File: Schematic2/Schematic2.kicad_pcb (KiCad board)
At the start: 2 copper layers, 100 x 119 mm, 52 parts, among them SW1 Rotary_Encoder_Switch, U1 Kailhlowprofile, U10 Kailhlowprofile, U11 Kailhlowprofile, U12 Kailhlowprofile, U13 Kailhlowprofile, U14 Kailhlowprofile, U15 Kailhlowprofile, U16 Kailhlowprofile, U17 Kailhlowprofile, U18 Kailhlowprofile, U19 Kailhlowprofile, U2 Kailhlowprofile, U20 Kailhlowprofile, U3 Kailhlowprofile, U4 Kailhlowprofile, U5 Kailhlowprofile, U6 Kailhlowprofile, U7 Kailhlowprofile, U8 Kailhlowprofile, U9 Kailhlowprofile

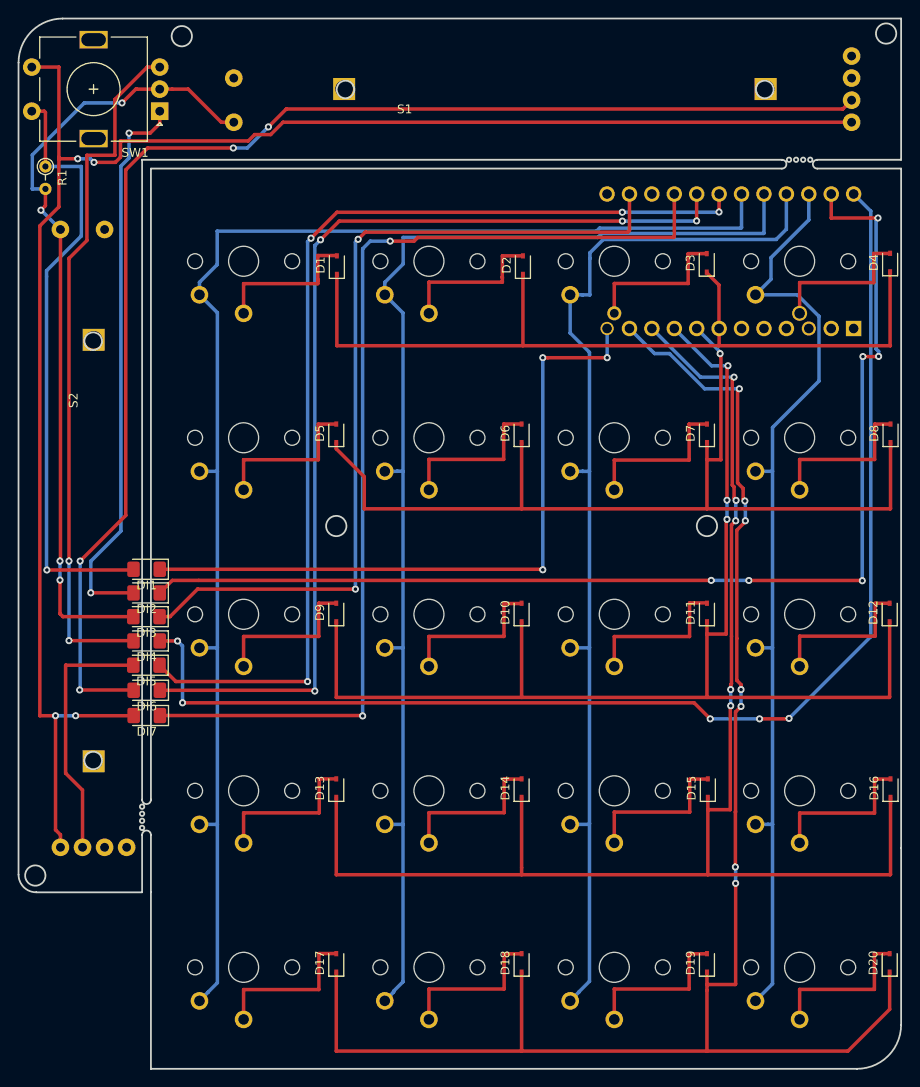
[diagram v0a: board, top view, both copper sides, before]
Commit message: Print time - final and absolutely done edition
This edition is completely done, for realz, and has all the files you need to print a macro keyboard with Kailh switches.
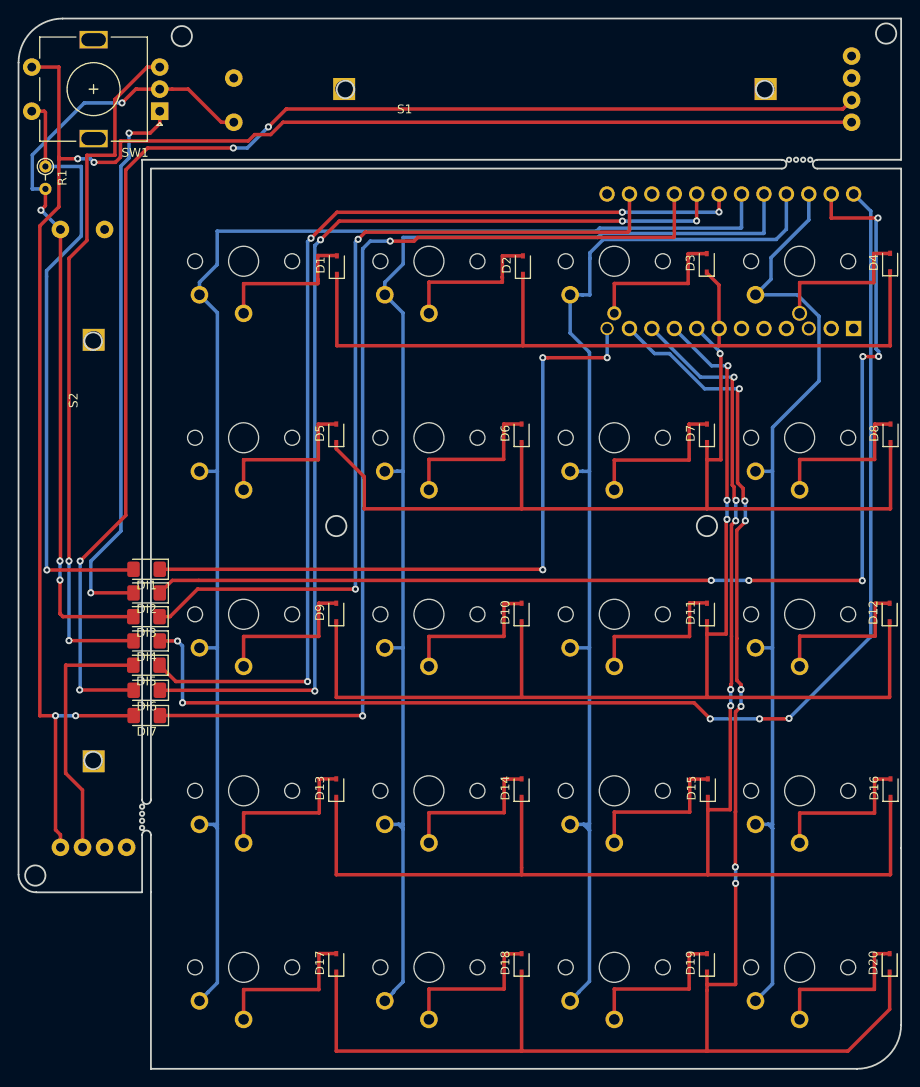
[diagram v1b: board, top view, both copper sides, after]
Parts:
- added G***: LOGO, Schematic2:AI_MF_D11Neg, B.Cu at (85.1, 104.1)
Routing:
- net C3: track 122.8 -> 123.8 mm
- net C2: track 140.9 -> 141.6 mm
- net C4: track 108.5 -> 109.1 mm
- net C1: track 159.2 -> 159.8 mm
